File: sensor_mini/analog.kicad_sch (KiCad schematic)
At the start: 7 parts, among them J2 Thermistor_conn, J3 Tank_pressure_conn

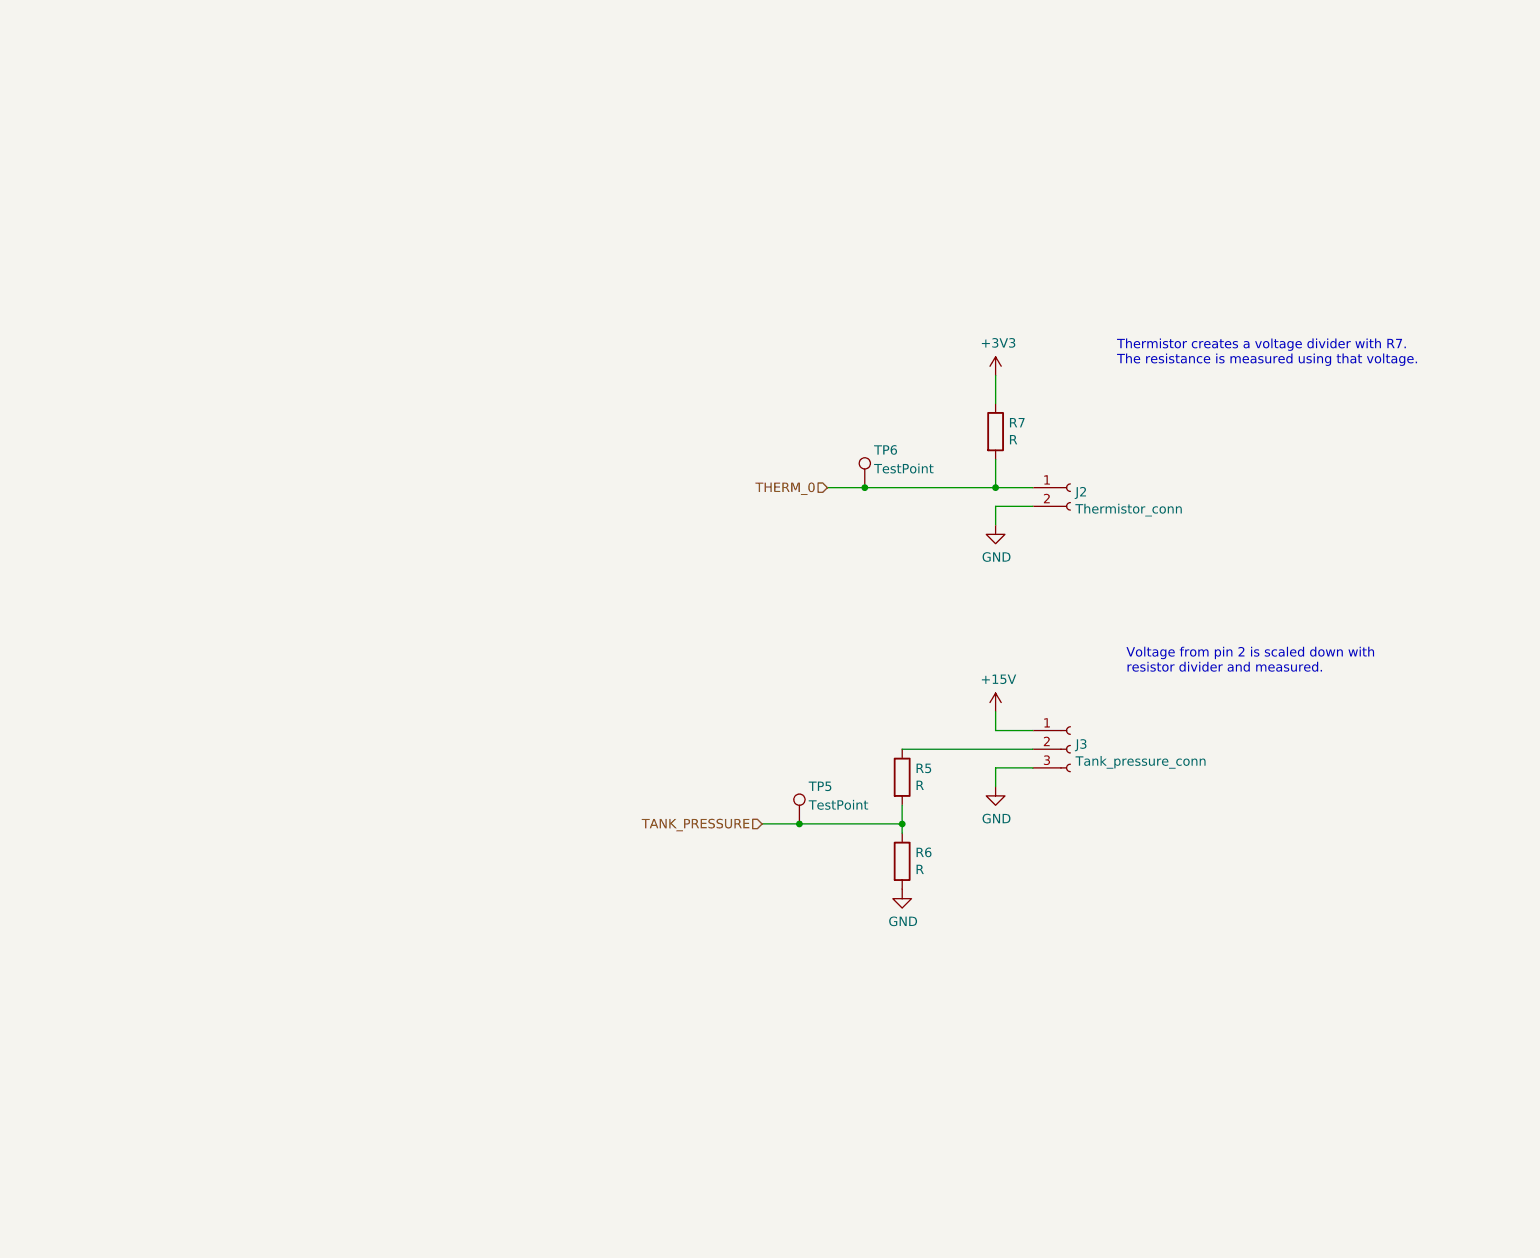
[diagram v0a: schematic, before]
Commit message: ICM-20948
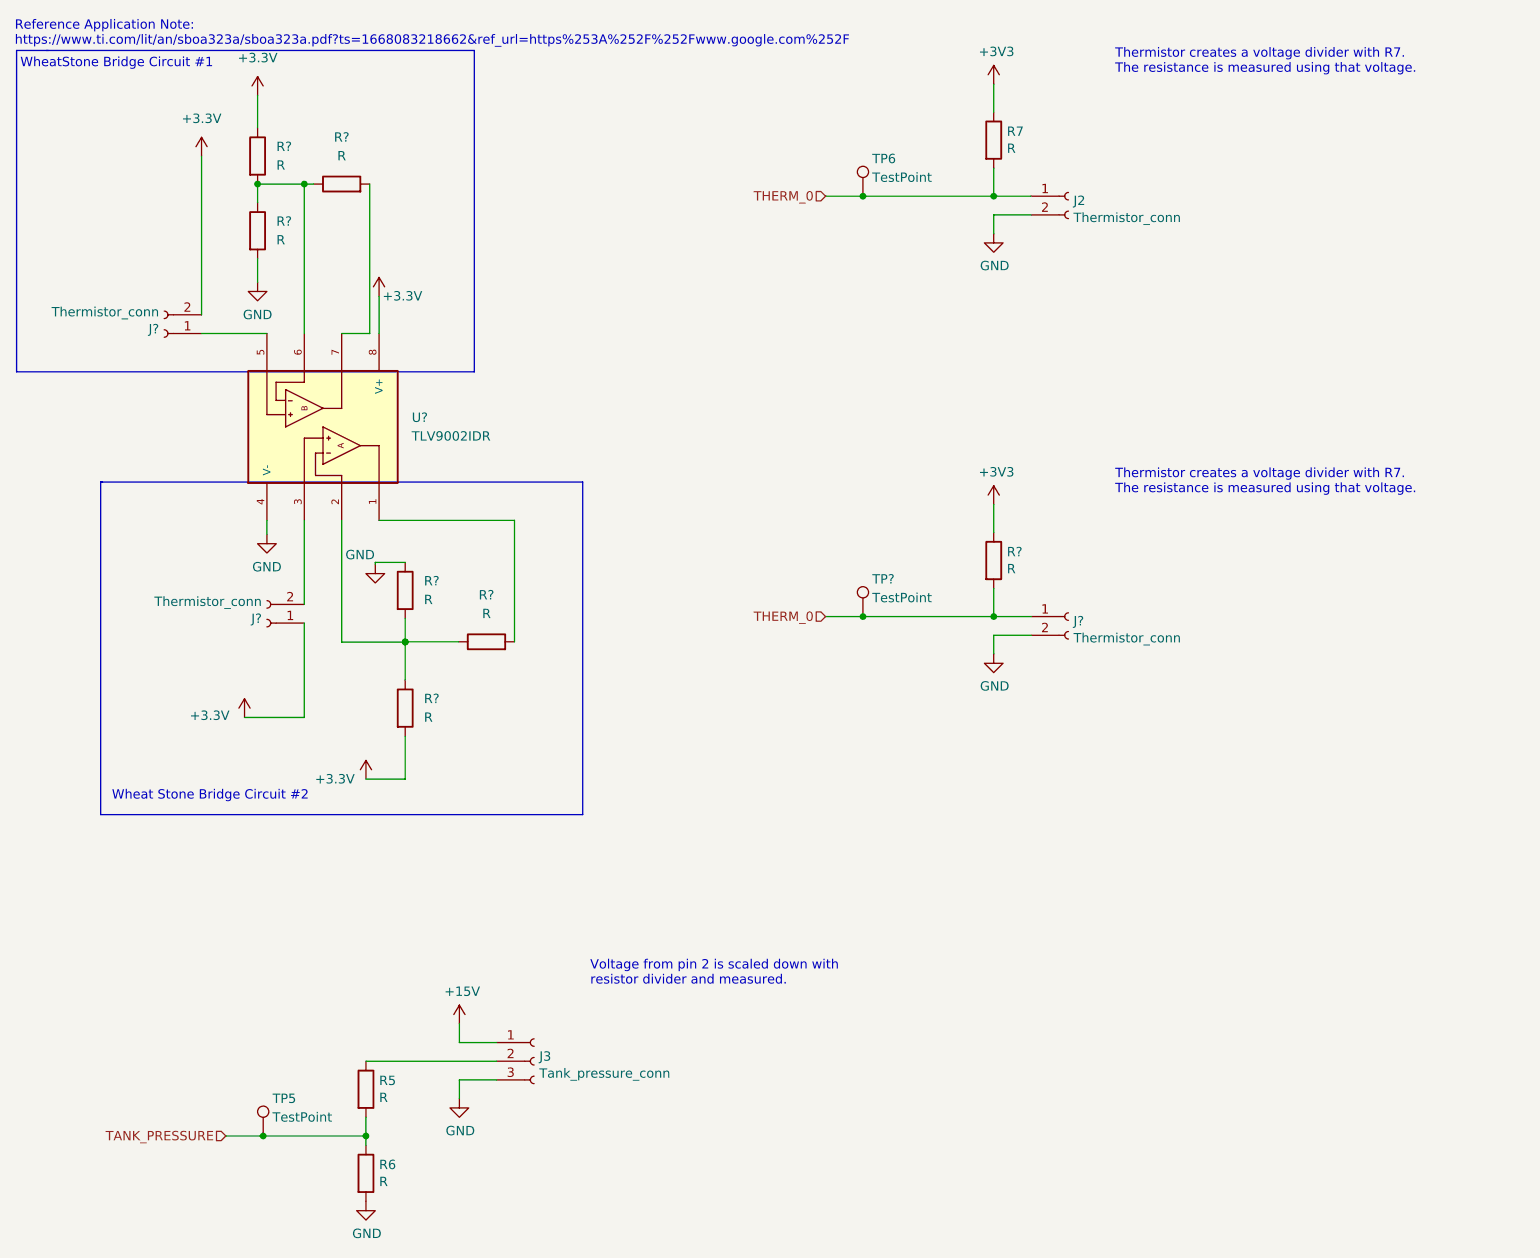
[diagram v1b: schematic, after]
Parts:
- added J? (x3): Thermistor_conn, Connector_JST:JST_PH_S2B-PH-K_1x02_P2.00mm_Horizontal, symbol sensors-rescue:Conn_01x02_Female-Connector
- added R? (x6): R, symbol Device:R
- added R?: R, Resistor_SMD:R_0805_2012Metric_Pad1.15x1.40mm_HandSolder, symbol Device:R
- added TP?: TestPoint, TestPoint:TestPoint_THTPad_2.0x2.0mm_Drill1.0mm, symbol Connector:TestPoint
- added U?: TLV9002IDR, SOIC127P599X175-8N, symbol TLV9002IDR:TLV9002IDR
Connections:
- net +3V3: now also R?.1
- net GND: now also J?.2 (Pin_2), R?.1, R?.2, U?.4 (V-)
- net THERM_0: now also J?.1 (Pin_1), R?.2, TP?.1
- new net: R?.1, R?.1, R?.2, U?.2
- new net: R?.1, R?.1, R?.2, U?.6
- new net: R?.2, U?.7
- new net: J?.1 (Pin_1), U?.5
- new net: R?.2, U?.1
- new net: J?.2 (Pin_2), U?.3
- new net +3.3V: J?.1 (Pin_1), J?.2 (Pin_2), R?.1, R?.2, U?.8 (V+)
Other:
- note added: "Reference Application Note: https://www.ti.com/lit/an/sboa323a/sboa323a.pdf?ts=1668083218662&ref_url=https%253A%252F%252Fwww.google.com%252F"
- note added: "Wheat Stone Bridge Circuit #2"
- note added: "WheatStone Bridge Circuit #1"
- moved on the sheet: J2, J3, R5, R6, R7, TP5, TP6
